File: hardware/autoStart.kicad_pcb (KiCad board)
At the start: 2 copper layers, 21 parts, among them J1 AudioJack3_Switch, J2 Screw_Terminal_01x03, Q1 BC547, U1 ICL7621BMTV, U2 ICL7621BMTV, U3 78S05M

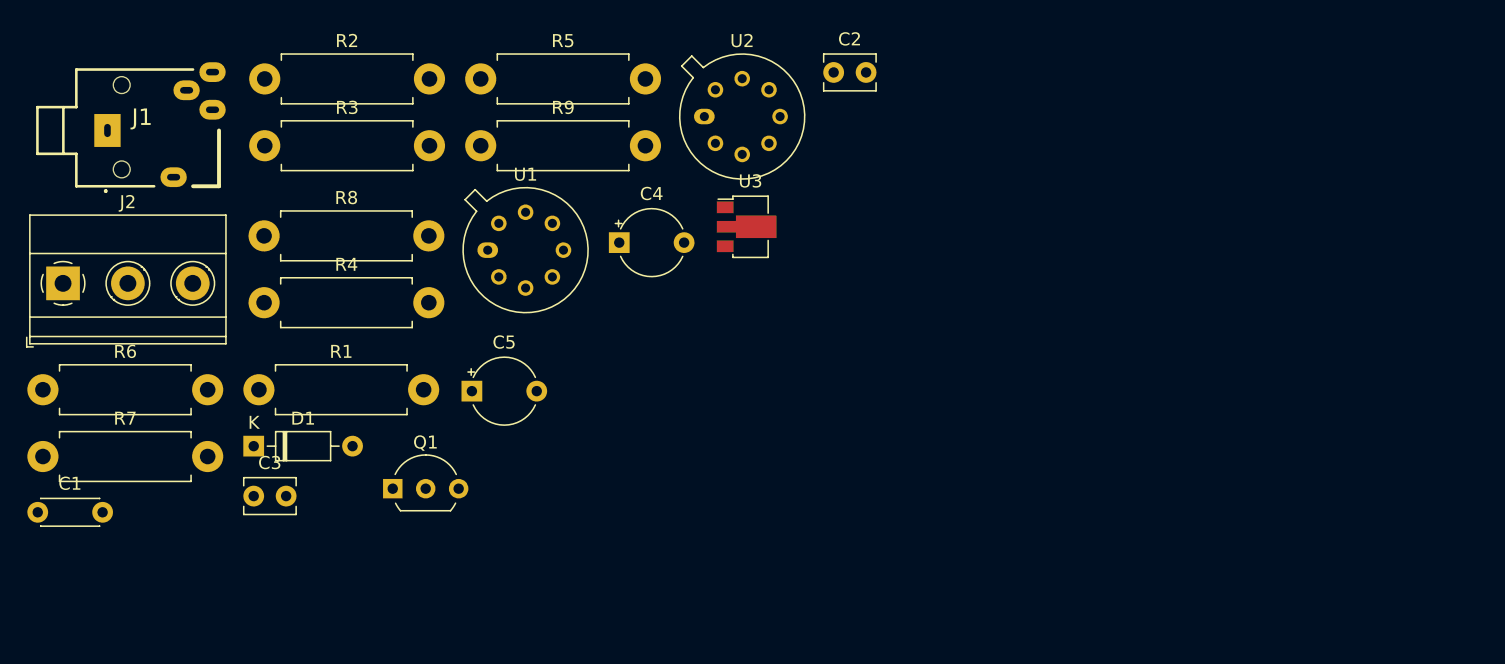
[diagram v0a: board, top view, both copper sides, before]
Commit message: SMD Mounts Initial commit
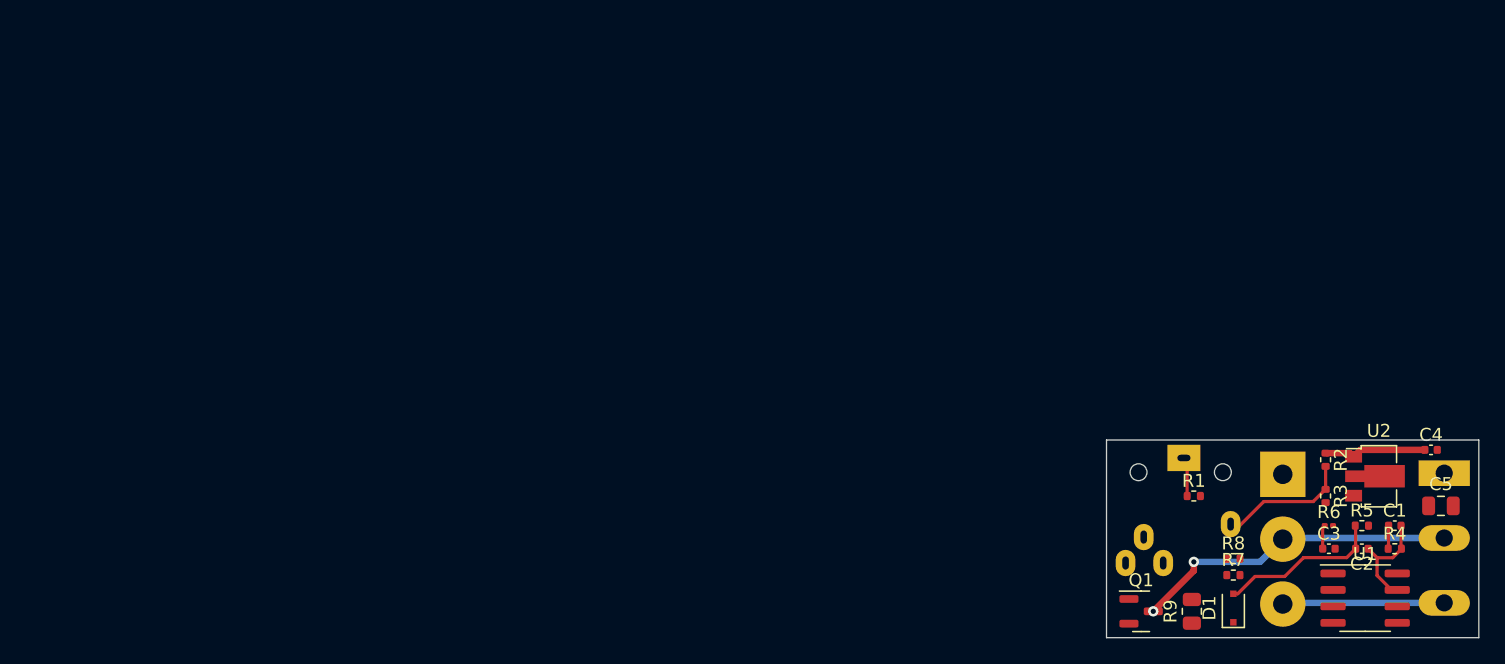
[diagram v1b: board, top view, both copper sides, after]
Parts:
- removed U3: 78S05M, Package_TO_SOT_SMD:SOT-89-3
- added J3: Conn_01x03_Male, Local_Project_Connectors_Library:PinHeader_1x03_P_5mm_Vertical-(Backside_Mount), F.Cu at (176.8, 71.0)
- C1: value 10nf -> C10nf_SMD; footprint Capacitor_THT:C_Disc_D4.3mm_W1.9mm_P5.00mm -> Capacitor_SMD:C_0402_1005Metric
- C2, C3: value 100nf -> C100nf_SMD; footprint Capacitor_THT:C_Disc_D3.8mm_W2.6mm_P2.50mm -> Capacitor_SMD:C_0402_1005Metric
- C4: value 0,1uf -> C100nf_SMD; footprint Capacitor_THT:CP_Radial_Tantal_D5.0mm_P5.00mm -> Capacitor_SMD:C_0402_1005Metric
- C5: value 0,47uf -> C330nf_SMD; footprint Capacitor_THT:CP_Radial_Tantal_D5.0mm_P5.00mm -> Capacitor_SMD:C_0805_2012Metric
- D1: value 1N4148 -> 1N4148WS; footprint Diode_THT:D_DO-35_SOD27_P7.62mm_Horizontal -> Diode_SMD:D_SOD-323F
- J1: footprint Local_Connectors:AUDIO_JACK_ASJ-195-L-HT -> Local_Connectors:AUDIO_JACK_ASJ-195-L-HT-(Backside_Mount)
- J2: value Screw_Terminal_01x03 -> Screw_Terminal_01x03-Connector; footprint TerminalBlock_Phoenix:TerminalBlock_Phoenix_MKDS-1,5-3_1x03_P5.00mm_Horizontal -> Local_Connectors:Phoenix_TERM_BLOCK_3POS_45DEG_5MM_PCB
- Q1: value BC547 -> S8050_SOT23; footprint Package_TO_SOT_THT:TO-92L_Inline_Wide -> Package_TO_SOT_SMD:SOT-23
- R1, R2, R3: value 10k -> R10K_0.0625W; footprint Resistor_THT:R_Axial_DIN0411_L9.9mm_D3.6mm_P12.70mm_Horizontal -> Resistor_SMD:R_0402_1005Metric
- R4: value 330k -> R330K_0.0625W; footprint Resistor_THT:R_Axial_DIN0411_L9.9mm_D3.6mm_P12.70mm_Horizontal -> Resistor_SMD:R_0402_1005Metric
- R5: value 100k -> R100K_0.0625W; footprint Resistor_THT:R_Axial_DIN0411_L9.9mm_D3.6mm_P12.70mm_Horizontal -> Resistor_SMD:R_0402_1005Metric
- R6: value 680k -> R680K_0.1W; footprint Resistor_THT:R_Axial_DIN0411_L9.9mm_D3.6mm_P12.70mm_Horizontal -> Resistor_SMD:R_0201_0603Metric
- R7: value 150k -> R150K_0.0625W; footprint Resistor_THT:R_Axial_DIN0411_L9.9mm_D3.6mm_P12.70mm_Horizontal -> Resistor_SMD:R_0402_1005Metric
- R8: value 33k -> R33K_0.0625W; footprint Resistor_THT:R_Axial_DIN0411_L9.9mm_D3.6mm_P12.70mm_Horizontal -> Resistor_SMD:R_0402_1005Metric
- R9: value 180 -> R180_0.125W; footprint Resistor_THT:R_Axial_DIN0411_L9.9mm_D3.6mm_P12.70mm_Horizontal -> Resistor_SMD:R_0805_2012Metric
- U1: value ICL7621BMTV -> LM358DR2G; footprint Package_TO_SOT_THT:TO-99-8 -> Package_SO:SOIC-8_3.9x4.9mm_P1.27mm
- U2: value ICL7621BMTV -> 78L05G_SOT89; footprint Package_TO_SOT_THT:TO-99-8 -> Package_TO_SOT_SMD:SOT-89-3
- moved J2 107.5 mm to (189.2, 70.9), turned to -90 degrees
- moved C1 104.6 mm to (185.4, 74.9)
- moved R6 99.7 mm to (180.3, 74.9)
- moved R7 92.2 mm to (173.0, 78.7)
- moved R4 89.2 mm to (185.4, 76.7)
- moved J1 88.4 mm to (169.2, 67.3), turned to 90 degrees
- moved R2 86.9 mm to (180.1, 69.8), turned to -90 degrees
- moved R3 86.1 mm to (180.1, 72.6), turned to -90 degrees
- moved C3 83.0 mm to (180.3, 76.7)
- moved R8 78.8 mm to (173.0, 77.5)
- moved D1 76.5 mm to (173.0, 81.3), turned to 90 degrees
- moved R5 76.2 mm to (182.9, 74.9)
- moved C5 75.2 mm to (189.0, 73.4)
- moved U1 72.8 mm to (183.1, 80.5)
- moved R1 72.5 mm to (169.9, 72.6)
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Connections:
- Q1 pad 1: Net-(J2-Pad2) -> Net-(Q1-Pad1)
- Q1 pad 2: Net-(Q1-Pad2) -> GND
- Q1 pad 3: GND -> Net-(J2-Pad2)
- R2 pad 1: Net-(J1-Pad2) -> VCC
- R2 pad 2: VCC -> Net-(J1-Pad2)
- R3 pad 1: GND -> Net-(J1-Pad2)
- R3 pad 2: Net-(J1-Pad2) -> GND
- R5 pad 1: GND -> Net-(C2-Pad2)
- R5 pad 2: Net-(C2-Pad2) -> GND
- R6 pad 1: GND -> Net-(C3-Pad1)
- R6 pad 2: Net-(C3-Pad1) -> GND
- R7 pad 1: Net-(R7-Pad1) -> VCC
- R7 pad 2: VCC -> Net-(R7-Pad2)
- R8 pad 1: GND -> Net-(R7-Pad2)
- R8 pad 2: Net-(R7-Pad1) -> GND
- R9 pad 1: Net-(Q1-Pad2) -> Net-(R9-Pad1)
- R9 pad 2: Net-(R9-Pad2) -> Net-(Q1-Pad1)
- U1 pad 1: Net-(C1-Pad2) -> Net-(R9-Pad1)
- U1 pad 2: Net-(J1-Pad2) -> Net-(R7-Pad2)
- U1 pad 3: Net-(C1-Pad1) -> Net-(C3-Pad1)
- U1 pad 4: (no net) -> GND
- U1 pad 5: Net-(C3-Pad1) -> Net-(C1-Pad1)
- U1 pad 6: Net-(R7-Pad1) -> Net-(J1-Pad2)
- U1 pad 7: Net-(R9-Pad2) -> Net-(C1-Pad2)
- U1 pad 8: (no net) -> VCC
- U2 pad 1: (no net) -> VCC
- U2 pad 2: (no net) -> GND
- U2 pad 3: (no net) -> VS
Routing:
- net Net-(J2-Pad2): track 0.00 -> 25.2 mm, vias 0 -> 2
- net VS: track 0.00 -> 14.2 mm
- net Net-(C2-Pad2): track 0.00 -> 12.7 mm
- net Net-(J1-Pad2): track 0.00 -> 10.2 mm
- net Net-(C1-Pad2): track 0.00 -> 8.33 mm
- net VCC: track 0.00 -> 7.98 mm
- net Net-(J1-Pad1): track 0.00 -> 2.36 mm
- net Net-(C3-Pad1): track 0.00 -> 1.84 mm
- net Net-(C1-Pad1): track 0.00 -> 1.79 mm
- net GND: track 0.00 -> 0.98 mm
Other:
- board outline added: 28.7 x 15.2 mm
